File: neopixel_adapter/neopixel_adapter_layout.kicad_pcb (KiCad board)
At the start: 2 copper layers, 91.4 x 81.3 mm, 480 parts, among them J1 Conn_01x02, J2 Conn_01x02

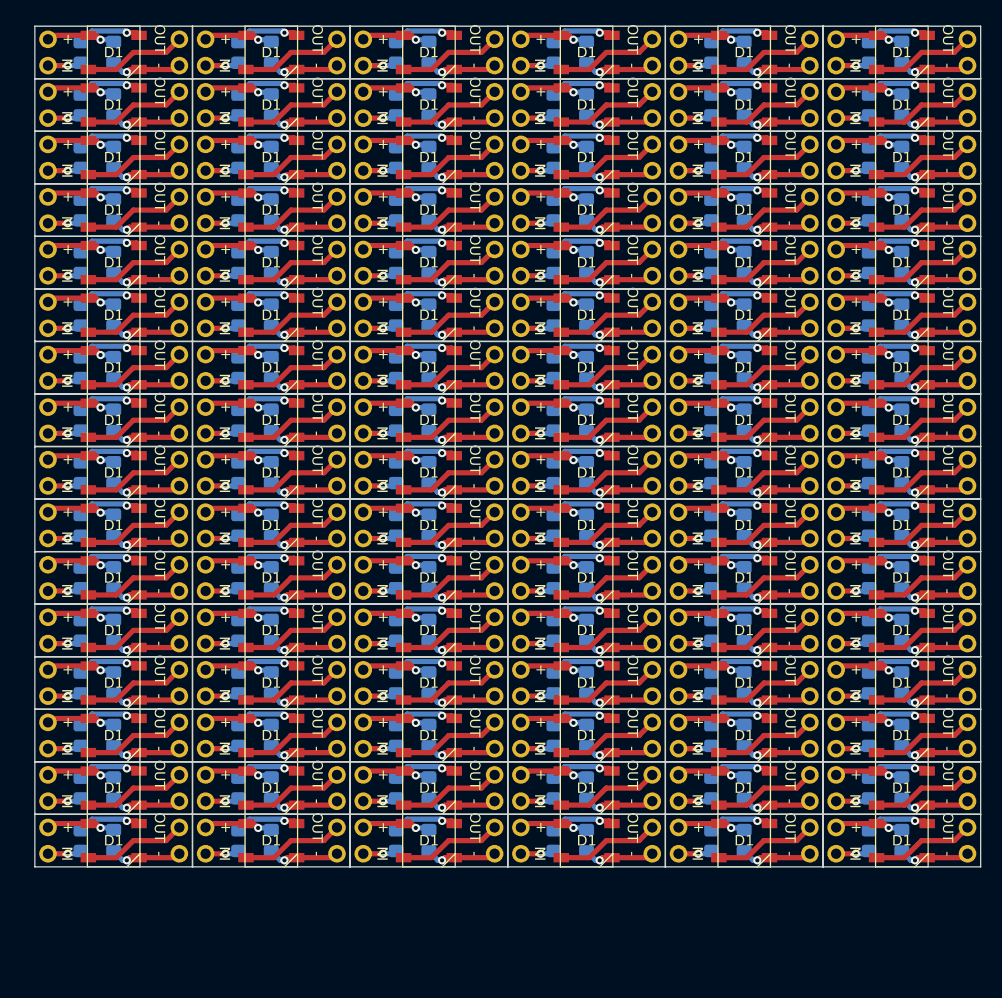
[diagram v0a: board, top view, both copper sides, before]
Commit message: Add .gitignore.
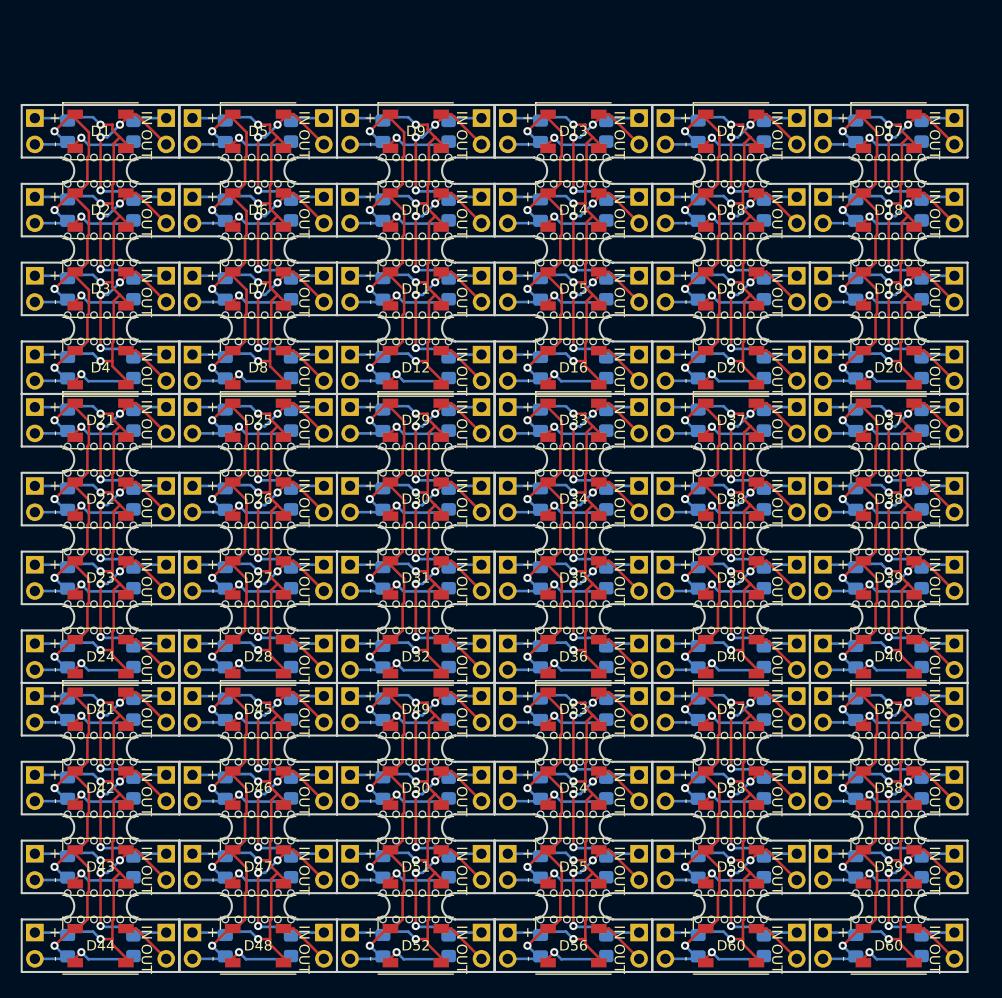
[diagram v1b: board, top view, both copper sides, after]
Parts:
- removed the C1 at (196.8, 68.6)
- removed the C1 at (166.4, 134.6)
- removed the C1 at (151.1, 124.5)
- removed the C1 at (196.8, 144.8)
- removed the C1 at (212.1, 104.1)
- removed the C1 at (181.6, 88.9)
- removed the C1 at (196.8, 139.7)
- removed the C1 at (212.1, 139.7)
- removed the C1 at (212.1, 78.7)
- removed the C1 at (135.9, 94.0)
- removed the C1 at (212.1, 124.5)
- removed the C1 at (181.6, 94.0)
- removed the C1 at (181.6, 129.5)
- removed the C1 at (151.1, 68.6)
- removed the C1 at (166.4, 114.3)
- removed the C1 at (212.1, 83.8)
- removed the C1 at (196.8, 78.7)
- removed the C1 at (166.4, 88.9)
- removed the C1 at (196.8, 109.2)
- removed the C1 at (151.1, 139.7)
- removed the C1 at (212.1, 68.6)
- removed the C1 at (181.6, 73.7)
- removed the C1 at (196.8, 94.0)
- removed the C1 at (166.4, 78.7)
- removed the C1 at (196.8, 119.4)
- removed the C1 at (135.9, 68.6)
- removed the C1 at (212.1, 144.8)
- removed the C1 at (151.1, 119.4)
- removed the C1 at (181.6, 139.7)
- removed the C1 at (181.6, 78.7)
- removed the C1 at (181.6, 124.5)
- removed the C1 at (151.1, 134.6)
- removed the C1 at (212.1, 99.1)
- removed the C1 at (212.1, 119.4)
- removed the C1 at (196.8, 114.3)
- removed the C1 at (212.1, 109.2)
- removed the C1 at (166.4, 109.2)
- removed the C1 at (212.1, 129.5)
- removed the C1 at (135.9, 78.7)
- removed the C1 at (151.1, 78.7)
- removed the C1 at (135.9, 124.5)
- removed the C1 at (196.8, 129.5)
- removed the C1 at (135.9, 144.8)
- removed the C1 at (181.6, 114.3)
- removed the C1 at (181.6, 99.1)
- removed the C1 at (166.4, 124.5)
- removed the C1 at (181.6, 119.4)
- removed the C1 at (166.4, 99.1)
- removed the C1 at (151.1, 88.9)
- removed the C1 at (196.8, 83.8)
- removed the C1 at (166.4, 129.5)
- removed the C1 at (166.4, 139.7)
- removed the C1 at (166.4, 119.4)
- removed the C1 at (181.6, 134.6)
- removed the C1 at (166.4, 83.8)
- removed the C1 at (135.9, 73.7)
- removed the C1 at (151.1, 73.7)
- removed the C1 at (196.8, 88.9)
- removed the C1 at (181.6, 104.1)
- removed the C1 at (135.9, 99.1)
- removed the C1 at (135.9, 109.2)
- removed the C1 at (151.1, 109.2)
- removed the C1 at (166.4, 68.6)
- removed the C1 at (196.8, 134.6)
- removed the C1 at (212.1, 88.9)
- removed the C1 at (212.1, 114.3)
- removed the C1 at (151.1, 99.1)
- removed the C1 at (151.1, 94.0)
- removed the C1 at (135.9, 139.7)
- removed the C1 at (151.1, 144.8)
- removed the C1 at (151.1, 83.8)
- removed the C1 at (135.9, 134.6)
- removed the C1 at (135.9, 83.8)
- removed the C1 at (196.8, 124.5)
- removed the C1 at (135.9, 88.9)
- removed the C1 at (151.1, 129.5)
- removed the C1 at (181.6, 144.8)
- removed the C1 at (135.9, 129.5)
- removed the C1 at (212.1, 94.0)
- removed the C1 at (212.1, 134.6)
- removed the C1 at (212.1, 73.7)
- removed the C1 at (135.9, 119.4)
- removed the C1 at (166.4, 94.0)
- removed the C1 at (181.6, 83.8)
- removed the C1 at (166.4, 144.8)
- removed the C1 at (151.1, 114.3)
- removed the C1 at (166.4, 104.1)
- removed the C1 at (181.6, 109.2)
- removed the C1 at (135.9, 114.3)
- removed the C1 at (151.1, 104.1)
- removed the C1 at (196.8, 99.1)
- removed the C1 at (196.8, 73.7)
- removed the C1 at (196.8, 104.1)
- removed the C1 at (181.6, 68.6)
- removed the C1 at (166.4, 73.7)
- removed the C1 at (135.9, 104.1)
- removed the D1 at (166.4, 68.6)
- removed the D1 at (135.9, 94.0)
- removed the D1 at (181.6, 88.9)
- removed the D1 at (135.9, 139.7)
- removed the D1 at (135.9, 124.5)
- removed the D1 at (181.6, 94.0)
- removed the D1 at (196.8, 144.8)
- removed the D1 at (181.6, 134.6)
- removed the D1 at (135.9, 129.5)
- removed the D1 at (166.4, 78.7)
- removed the D1 at (135.9, 134.6)
- removed the D1 at (135.9, 99.1)
- removed the D1 at (135.9, 88.9)
- removed the D1 at (166.4, 139.7)
- removed the D1 at (196.8, 139.7)
- removed the D1 at (212.1, 139.7)
- removed the D1 at (151.1, 78.7)
- removed the D1 at (196.8, 73.7)
- removed the D1 at (166.4, 109.2)
- removed the D1 at (166.4, 94.0)
- removed the D1 at (166.4, 114.3)
- removed the D1 at (166.4, 119.4)
- removed the D1 at (166.4, 83.8)
- removed the D1 at (181.6, 99.1)
- removed the D1 at (196.8, 114.3)
- removed the D1 at (196.8, 68.6)
- removed the D1 at (181.6, 109.2)
- removed the D1 at (181.6, 144.8)
- removed the D1 at (181.6, 78.7)
- removed the D1 at (212.1, 144.8)
- removed the D1 at (151.1, 68.6)
- removed the D1 at (196.8, 124.5)
- removed the D1 at (212.1, 119.4)
- removed the D1 at (135.9, 73.7)
- removed the D1 at (212.1, 68.6)
- removed the D1 at (151.1, 129.5)
- removed the D1 at (196.8, 104.1)
- removed the D1 at (151.1, 83.8)
- removed the D1 at (151.1, 104.1)
- removed the D1 at (181.6, 114.3)
- removed the D1 at (181.6, 73.7)
- removed the D1 at (212.1, 109.2)
- removed the D1 at (135.9, 104.1)
- removed the D1 at (166.4, 129.5)
- removed the D1 at (196.8, 94.0)
- removed the D1 at (196.8, 88.9)
- removed the D1 at (166.4, 144.8)
- removed the D1 at (196.8, 83.8)
- removed the D1 at (166.4, 73.7)
- removed the D1 at (212.1, 114.3)
- removed the D1 at (135.9, 68.6)
- removed the D1 at (181.6, 83.8)
- removed the D1 at (135.9, 144.8)
- removed the D1 at (196.8, 119.4)
- removed the D1 at (212.1, 104.1)
- removed the D1 at (196.8, 109.2)
- removed the D1 at (151.1, 94.0)
- removed the D1 at (212.1, 88.9)
- removed the D1 at (196.8, 129.5)
- removed the D1 at (151.1, 114.3)
- removed the D1 at (151.1, 119.4)
- removed the D1 at (135.9, 114.3)
- removed the D1 at (181.6, 119.4)
- removed the D1 at (151.1, 134.6)
- removed the D1 at (212.1, 124.5)
- removed the D1 at (166.4, 88.9)
- removed the D1 at (181.6, 104.1)
- removed the D1 at (212.1, 73.7)
- removed the D1 at (166.4, 99.1)
- removed the D1 at (181.6, 139.7)
- removed the D1 at (212.1, 83.8)
- removed the D1 at (151.1, 139.7)
- removed the D1 at (135.9, 83.8)
- removed the D1 at (212.1, 78.7)
- removed the D1 at (151.1, 109.2)
- removed the D1 at (166.4, 104.1)
- removed the D1 at (212.1, 129.5)
- removed the D1 at (151.1, 144.8)
- removed the D1 at (151.1, 124.5)
- removed the D1 at (135.9, 109.2)
- removed the D1 at (151.1, 88.9)
- removed the D1 at (151.1, 99.1)
- removed the D1 at (135.9, 78.7)
- removed the D1 at (196.8, 134.6)
- removed the D1 at (212.1, 134.6)
- removed the D1 at (181.6, 68.6)
- removed the D1 at (181.6, 129.5)
- removed the D1 at (135.9, 119.4)
- removed the D1 at (212.1, 99.1)
- removed the D1 at (212.1, 94.0)
- removed the D1 at (196.8, 78.7)
- removed the D1 at (181.6, 124.5)
- removed the D1 at (166.4, 134.6)
- removed the D1 at (151.1, 73.7)
- removed the D1 at (166.4, 124.5)
- removed the D1 at (196.8, 99.1)
- removed the J1 at (190.5, 143.5)
- removed the J1 at (205.7, 92.7)
- removed the J1 at (160.0, 128.3)
- removed the J1 at (129.5, 82.5)
- removed the J1 at (175.3, 118.1)
- removed the J1 at (129.5, 118.1)
- removed the J1 at (190.5, 108.0)
- removed the J1 at (144.8, 102.9)
- removed the J1 at (205.7, 143.5)
- removed the J1 at (175.3, 123.2)
- removed the J1 at (205.7, 113.0)
- removed the J1 at (205.7, 77.5)
- removed the J1 at (175.3, 143.5)
- removed the J1 at (190.5, 97.8)
- removed the J1 at (160.0, 97.8)
- removed the J1 at (205.7, 108.0)
- removed the J1 at (129.5, 72.4)
- removed the J1 at (129.5, 92.7)
- removed the J1 at (144.8, 113.0)
- removed the J1 at (175.3, 128.3)
- removed the J1 at (129.5, 123.2)
- removed the J1 at (160.0, 87.6)
- removed the J1 at (160.0, 92.7)
- removed the J1 at (129.5, 128.3)
- removed the J1 at (205.7, 82.5)
- removed the J1 at (144.8, 77.5)
- removed the J1 at (144.8, 87.6)
- removed the J1 at (205.7, 97.8)
- removed the J1 at (190.5, 72.4)
- removed the J1 at (205.7, 138.4)
- removed the J1 at (175.3, 113.0)
- removed the J1 at (190.5, 102.9)
- removed the J1 at (144.8, 128.3)
- removed the J1 at (144.8, 92.7)
- removed the J1 at (160.0, 67.3)
- removed the J1 at (190.5, 123.2)
- removed the J1 at (144.8, 82.5)
- removed the J1 at (129.5, 143.5)
- removed the J1 at (129.5, 108.0)
- removed the J1 at (190.5, 138.4)
- removed the J1 at (175.3, 138.4)
- removed the J1 at (190.5, 67.3)
- removed the J1 at (205.7, 128.3)
- removed the J1 at (175.3, 82.5)
- removed the J1 at (129.5, 102.9)
- removed the J1 at (190.5, 92.7)
- removed the J1 at (205.7, 118.1)
- removed the J1 at (190.5, 113.0)
- removed the J1 at (144.8, 123.2)
- removed the J1 at (160.0, 113.0)
- removed the J1 at (175.3, 108.0)
- removed the J1 at (190.5, 133.3)
- removed the J1 at (190.5, 87.6)
- removed the J1 at (175.3, 87.6)
- removed the J1 at (160.0, 123.2)
- removed the J1 at (205.7, 133.3)
- removed the J1 at (160.0, 72.4)
- removed the J1 at (144.8, 108.0)
- removed the J1 at (175.3, 67.3)
- removed the J1 at (129.5, 138.4)
- removed the J1 at (205.7, 67.3)
- removed the J1 at (205.7, 72.4)
- removed the J1 at (160.0, 118.1)
- removed the J1 at (144.8, 72.4)
- removed the J1 at (129.5, 113.0)
- removed the J1 at (175.3, 97.8)
- removed the J1 at (144.8, 143.5)
- removed the J1 at (160.0, 108.0)
- removed the J1 at (190.5, 77.5)
- removed the J1 at (175.3, 92.7)
- removed the J1 at (205.7, 102.9)
- removed the J1 at (129.5, 133.3)
- removed the J1 at (175.3, 102.9)
- removed the J1 at (160.0, 82.5)
- removed the J1 at (129.5, 97.8)
- removed the J1 at (144.8, 118.1)
- removed the J1 at (175.3, 133.3)
- removed the J1 at (144.8, 133.3)
- removed the J1 at (190.5, 128.3)
- removed the J1 at (175.3, 77.5)
- removed the J1 at (190.5, 118.1)
- removed the J1 at (160.0, 102.9)
- removed the J1 at (205.7, 123.2)
- removed the J1 at (129.5, 77.5)
- removed the J1 at (129.5, 87.6)
- removed the J1 at (160.0, 77.5)
- removed the J1 at (129.5, 67.3)
- removed the J1 at (160.0, 138.4)
- removed the J1 at (160.0, 133.3)
- removed the J1 at (144.8, 97.8)
- removed the J1 at (175.3, 72.4)
- removed the J1 at (144.8, 67.3)
- removed the J1 at (160.0, 143.5)
- removed the J1 at (190.5, 82.5)
- removed the J1 at (144.8, 138.4)
- removed the J1 at (205.7, 87.6)
- removed the J2 at (172.7, 133.3)
- removed the J2 at (142.2, 97.8)
- removed the J2 at (218.4, 77.5)
- removed the J2 at (203.2, 97.8)
- removed the J2 at (172.7, 128.3)
- removed the J2 at (142.2, 123.2)
- removed the J2 at (142.2, 92.7)
- removed the J2 at (188.0, 67.3)
- removed the J2 at (157.5, 97.8)
- removed the J2 at (218.4, 102.9)
- removed the J2 at (157.5, 128.3)
- removed the J2 at (172.7, 108.0)
- removed the J2 at (172.7, 138.4)
- removed the J2 at (157.5, 143.5)
- removed the J2 at (157.5, 102.9)
- removed the J2 at (142.2, 138.4)
- removed the J2 at (157.5, 92.7)
- removed the J2 at (218.4, 138.4)
- removed the J2 at (218.4, 118.1)
- removed the J2 at (188.0, 72.4)
- removed the J2 at (218.4, 128.3)
- removed the J2 at (142.2, 82.5)
- removed the J2 at (157.5, 87.6)
- removed the J2 at (218.4, 82.5)
- removed the J2 at (172.7, 92.7)
- removed the J2 at (188.0, 97.8)
- removed the J2 at (218.4, 92.7)
- removed the J2 at (188.0, 138.4)
- removed the J2 at (172.7, 72.4)
- removed the J2 at (188.0, 143.5)
- removed the J2 at (203.2, 143.5)
- removed the J2 at (172.7, 82.5)
- removed the J2 at (142.2, 128.3)
- removed the J2 at (218.4, 123.2)
- removed the J2 at (172.7, 113.0)
- removed the J2 at (188.0, 92.7)
- removed the J2 at (203.2, 113.0)
- removed the J2 at (172.7, 87.6)
- removed the J2 at (203.2, 123.2)
- removed the J2 at (157.5, 113.0)
- removed the J2 at (157.5, 77.5)
- removed the J2 at (203.2, 77.5)
- removed the J2 at (203.2, 118.1)
- removed the J2 at (172.7, 77.5)
- removed the J2 at (142.2, 87.6)
- removed the J2 at (203.2, 138.4)
- removed the J2 at (218.4, 67.3)
- removed the J2 at (188.0, 108.0)
- removed the J2 at (188.0, 123.2)
- removed the J2 at (142.2, 113.0)
- removed the J2 at (218.4, 133.3)
- removed the J2 at (203.2, 108.0)
- removed the J2 at (172.7, 67.3)
- removed the J2 at (142.2, 72.4)
- removed the J2 at (203.2, 72.4)
- removed the J2 at (157.5, 108.0)
- removed the J2 at (142.2, 108.0)
- removed the J2 at (188.0, 128.3)
- removed the J2 at (203.2, 128.3)
- removed the J2 at (188.0, 133.3)
- removed the J2 at (157.5, 133.3)
- removed the J2 at (172.7, 118.1)
- removed the J2 at (188.0, 82.5)
- removed the J2 at (218.4, 97.8)
- removed the J2 at (203.2, 92.7)
- removed the J2 at (157.5, 82.5)
- removed the J2 at (218.4, 143.5)
- removed the J2 at (218.4, 87.6)
- removed the J2 at (142.2, 102.9)
- removed the J2 at (172.7, 143.5)
- removed the J2 at (188.0, 118.1)
- removed the J2 at (203.2, 133.3)
- removed the J2 at (157.5, 118.1)
- removed the J2 at (188.0, 102.9)
- removed the J2 at (172.7, 97.8)
- removed the J2 at (218.4, 113.0)
- removed the J2 at (157.5, 138.4)
- removed the J2 at (157.5, 72.4)
- removed the J2 at (142.2, 143.5)
- removed the J2 at (157.5, 123.2)
- removed the J2 at (218.4, 108.0)
- removed the J2 at (142.2, 133.3)
- removed the J2 at (203.2, 67.3)
- removed the J2 at (157.5, 67.3)
- removed the J2 at (203.2, 87.6)
- removed the J2 at (188.0, 77.5)
- removed the J2 at (172.7, 102.9)
- removed the J2 at (203.2, 102.9)
- removed the J2 at (218.4, 72.4)
- removed the J2 at (203.2, 82.5)
- removed the J2 at (142.2, 67.3)
- removed the J2 at (142.2, 77.5)
- removed the J2 at (172.7, 123.2)
- removed the J2 at (188.0, 113.0)
- removed the J2 at (142.2, 118.1)
- removed the J2 at (188.0, 87.6)
- removed the R1 at (178.4, 114.3)
- removed the R1 at (132.7, 99.1)
- removed the R1 at (193.7, 124.5)
- removed the R1 at (148.0, 94.0)
- removed the R1 at (178.4, 83.8)
- removed the R1 at (193.7, 94.0)
- removed the R1 at (163.2, 78.7)
- removed the R1 at (132.7, 114.3)
- removed the R1 at (178.4, 73.7)
- removed the R1 at (163.2, 144.8)
- removed the R1 at (193.7, 139.7)
- removed the R1 at (132.7, 88.9)
- removed the R1 at (148.0, 73.7)
- removed the R1 at (148.0, 68.6)
- removed the R1 at (178.4, 99.1)
- removed the R1 at (163.2, 104.1)
- removed the R1 at (193.7, 83.8)
- removed the R1 at (193.7, 114.3)
- removed the R1 at (178.4, 88.9)
- removed the R1 at (148.0, 134.6)
- removed the R1 at (132.7, 124.5)
- removed the R1 at (132.7, 68.6)
- removed the R1 at (178.4, 78.7)
- removed the R1 at (208.9, 83.8)
- removed the R1 at (208.9, 99.1)
- removed the R1 at (132.7, 94.0)
- removed the R1 at (208.9, 129.5)
- removed the R1 at (178.4, 144.8)
- removed the R1 at (132.7, 104.1)
- removed the R1 at (178.4, 134.6)
- removed the R1 at (193.7, 119.4)
- removed the R1 at (193.7, 134.6)
- removed the R1 at (208.9, 88.9)
- removed the R1 at (178.4, 139.7)
- removed the R1 at (163.2, 114.3)
- removed the R1 at (178.4, 124.5)
- removed the R1 at (132.7, 144.8)
- removed the R1 at (193.7, 144.8)
- removed the R1 at (163.2, 124.5)
- removed the R1 at (208.9, 119.4)
- removed the R1 at (178.4, 129.5)
- removed the R1 at (163.2, 73.7)
- removed the R1 at (163.2, 134.6)
- removed the R1 at (163.2, 83.8)
- removed the R1 at (208.9, 73.7)
- removed the R1 at (148.0, 124.5)
- removed the R1 at (178.4, 94.0)
- removed the R1 at (148.0, 114.3)
- removed the R1 at (163.2, 88.9)
- removed the R1 at (163.2, 129.5)
- removed the R1 at (208.9, 109.2)
- removed the R1 at (193.7, 109.2)
- removed the R1 at (178.4, 119.4)
- removed the R1 at (148.0, 129.5)
- removed the R1 at (193.7, 104.1)
- removed the R1 at (132.7, 73.7)
- removed the R1 at (148.0, 139.7)
- removed the R1 at (148.0, 99.1)
- removed the R1 at (208.9, 139.7)
- removed the R1 at (148.0, 104.1)
- removed the R1 at (178.4, 109.2)
- removed the R1 at (208.9, 68.6)
- removed the R1 at (193.7, 99.1)
- removed the R1 at (163.2, 68.6)
- removed the R1 at (193.7, 129.5)
- removed the R1 at (132.7, 109.2)
- removed the R1 at (193.7, 88.9)
- removed the R1 at (132.7, 129.5)
- removed the R1 at (132.7, 139.7)
- removed the R1 at (208.9, 134.6)
- removed the R1 at (148.0, 119.4)
- removed the R1 at (163.2, 119.4)
- removed the R1 at (193.7, 68.6)
- removed the R1 at (132.7, 78.7)
- removed the R1 at (193.7, 78.7)
- removed the R1 at (163.2, 94.0)
- removed the R1 at (178.4, 68.6)
- removed the R1 at (148.0, 78.7)
- removed the R1 at (163.2, 139.7)
- removed the R1 at (163.2, 109.2)
- removed the R1 at (178.4, 104.1)
- removed the R1 at (132.7, 83.8)
- removed the R1 at (208.9, 94.0)
- removed the R1 at (163.2, 99.1)
- removed the R1 at (148.0, 88.9)
- removed the R1 at (208.9, 124.5)
- removed the R1 at (148.0, 144.8)
- removed the R1 at (208.9, 144.8)
- removed the R1 at (132.7, 134.6)
- removed the R1 at (208.9, 78.7)
- removed the R1 at (148.0, 109.2)
- removed the R1 at (208.9, 104.1)
- removed the R1 at (132.7, 119.4)
- removed the R1 at (208.9, 114.3)
- removed the R1 at (193.7, 73.7)
- removed the R1 at (148.0, 83.8)
- added C1: 0.1uF, Capacitor_SMD:C_0805_2012Metric_Pad1.18x1.45mm_HandSolder, B.Cu at (131.4, 76.2)
- added C10: 0.1uF, Capacitor_SMD:C_0805_2012Metric_Pad1.18x1.45mm_HandSolder, B.Cu at (161.9, 83.8)
- added C11: 0.1uF, Capacitor_SMD:C_0805_2012Metric_Pad1.18x1.45mm_HandSolder, B.Cu at (161.9, 91.4)
- added C12: 0.1uF, Capacitor_SMD:C_0805_2012Metric_Pad1.18x1.45mm_HandSolder, B.Cu at (161.9, 99.1)
- added C13: 0.1uF, Capacitor_SMD:C_0805_2012Metric_Pad1.18x1.45mm_HandSolder, B.Cu at (177.2, 76.2)
- added C14: 0.1uF, Capacitor_SMD:C_0805_2012Metric_Pad1.18x1.45mm_HandSolder, B.Cu at (177.2, 83.8)
- added C15: 0.1uF, Capacitor_SMD:C_0805_2012Metric_Pad1.18x1.45mm_HandSolder, B.Cu at (177.2, 91.4)
- added C16: 0.1uF, Capacitor_SMD:C_0805_2012Metric_Pad1.18x1.45mm_HandSolder, B.Cu at (177.2, 99.1)
- added C17: 0.1uF, Capacitor_SMD:C_0805_2012Metric_Pad1.18x1.45mm_HandSolder, B.Cu at (207.6, 76.2)
- added C17: 0.1uF, Capacitor_SMD:C_0805_2012Metric_Pad1.18x1.45mm_HandSolder, B.Cu at (192.4, 76.2)
- added C18: 0.1uF, Capacitor_SMD:C_0805_2012Metric_Pad1.18x1.45mm_HandSolder, B.Cu at (192.4, 83.8)
- added C18: 0.1uF, Capacitor_SMD:C_0805_2012Metric_Pad1.18x1.45mm_HandSolder, B.Cu at (207.6, 83.8)
- added C19: 0.1uF, Capacitor_SMD:C_0805_2012Metric_Pad1.18x1.45mm_HandSolder, B.Cu at (207.6, 91.4)
- added C19: 0.1uF, Capacitor_SMD:C_0805_2012Metric_Pad1.18x1.45mm_HandSolder, B.Cu at (192.4, 91.4)
- added C2: 0.1uF, Capacitor_SMD:C_0805_2012Metric_Pad1.18x1.45mm_HandSolder, B.Cu at (131.4, 83.8)
- added C20: 0.1uF, Capacitor_SMD:C_0805_2012Metric_Pad1.18x1.45mm_HandSolder, B.Cu at (207.6, 99.1)
- added C20: 0.1uF, Capacitor_SMD:C_0805_2012Metric_Pad1.18x1.45mm_HandSolder, B.Cu at (192.4, 99.1)
- added C21: 0.1uF, Capacitor_SMD:C_0805_2012Metric_Pad1.18x1.45mm_HandSolder, B.Cu at (131.4, 104.1)
- added C22: 0.1uF, Capacitor_SMD:C_0805_2012Metric_Pad1.18x1.45mm_HandSolder, B.Cu at (131.4, 111.8)
- added C23: 0.1uF, Capacitor_SMD:C_0805_2012Metric_Pad1.18x1.45mm_HandSolder, B.Cu at (131.4, 119.4)
- added C24: 0.1uF, Capacitor_SMD:C_0805_2012Metric_Pad1.18x1.45mm_HandSolder, B.Cu at (131.4, 127.0)
- added C25: 0.1uF, Capacitor_SMD:C_0805_2012Metric_Pad1.18x1.45mm_HandSolder, B.Cu at (146.7, 104.1)
- added C26: 0.1uF, Capacitor_SMD:C_0805_2012Metric_Pad1.18x1.45mm_HandSolder, B.Cu at (146.7, 111.8)
- added C27: 0.1uF, Capacitor_SMD:C_0805_2012Metric_Pad1.18x1.45mm_HandSolder, B.Cu at (146.7, 119.4)
- added C28: 0.1uF, Capacitor_SMD:C_0805_2012Metric_Pad1.18x1.45mm_HandSolder, B.Cu at (146.7, 127.0)
- added C29: 0.1uF, Capacitor_SMD:C_0805_2012Metric_Pad1.18x1.45mm_HandSolder, B.Cu at (161.9, 104.1)
- added C3: 0.1uF, Capacitor_SMD:C_0805_2012Metric_Pad1.18x1.45mm_HandSolder, B.Cu at (131.4, 91.4)
- added C30: 0.1uF, Capacitor_SMD:C_0805_2012Metric_Pad1.18x1.45mm_HandSolder, B.Cu at (161.9, 111.8)
- added C31: 0.1uF, Capacitor_SMD:C_0805_2012Metric_Pad1.18x1.45mm_HandSolder, B.Cu at (161.9, 119.4)
- added C32: 0.1uF, Capacitor_SMD:C_0805_2012Metric_Pad1.18x1.45mm_HandSolder, B.Cu at (161.9, 127.0)
- added C33: 0.1uF, Capacitor_SMD:C_0805_2012Metric_Pad1.18x1.45mm_HandSolder, B.Cu at (177.2, 104.1)
- added C34: 0.1uF, Capacitor_SMD:C_0805_2012Metric_Pad1.18x1.45mm_HandSolder, B.Cu at (177.2, 111.8)
- added C35: 0.1uF, Capacitor_SMD:C_0805_2012Metric_Pad1.18x1.45mm_HandSolder, B.Cu at (177.2, 119.4)
- added C36: 0.1uF, Capacitor_SMD:C_0805_2012Metric_Pad1.18x1.45mm_HandSolder, B.Cu at (177.2, 127.0)
- added C37: 0.1uF, Capacitor_SMD:C_0805_2012Metric_Pad1.18x1.45mm_HandSolder, B.Cu at (207.6, 104.1)
- added C37: 0.1uF, Capacitor_SMD:C_0805_2012Metric_Pad1.18x1.45mm_HandSolder, B.Cu at (192.4, 104.1)
- added C38: 0.1uF, Capacitor_SMD:C_0805_2012Metric_Pad1.18x1.45mm_HandSolder, B.Cu at (192.4, 111.8)
- added C38: 0.1uF, Capacitor_SMD:C_0805_2012Metric_Pad1.18x1.45mm_HandSolder, B.Cu at (207.6, 111.8)
- added C39: 0.1uF, Capacitor_SMD:C_0805_2012Metric_Pad1.18x1.45mm_HandSolder, B.Cu at (192.4, 119.4)
- added C39: 0.1uF, Capacitor_SMD:C_0805_2012Metric_Pad1.18x1.45mm_HandSolder, B.Cu at (207.6, 119.4)
- added C4: 0.1uF, Capacitor_SMD:C_0805_2012Metric_Pad1.18x1.45mm_HandSolder, B.Cu at (131.4, 99.1)
- added C40: 0.1uF, Capacitor_SMD:C_0805_2012Metric_Pad1.18x1.45mm_HandSolder, B.Cu at (207.6, 127.0)
- added C40: 0.1uF, Capacitor_SMD:C_0805_2012Metric_Pad1.18x1.45mm_HandSolder, B.Cu at (192.4, 127.0)
- added C41: 0.1uF, Capacitor_SMD:C_0805_2012Metric_Pad1.18x1.45mm_HandSolder, B.Cu at (131.4, 132.1)
- added C42: 0.1uF, Capacitor_SMD:C_0805_2012Metric_Pad1.18x1.45mm_HandSolder, B.Cu at (131.4, 139.7)
- added C43: 0.1uF, Capacitor_SMD:C_0805_2012Metric_Pad1.18x1.45mm_HandSolder, B.Cu at (131.4, 147.3)
- added C44: 0.1uF, Capacitor_SMD:C_0805_2012Metric_Pad1.18x1.45mm_HandSolder, B.Cu at (131.4, 154.9)
- added C45: 0.1uF, Capacitor_SMD:C_0805_2012Metric_Pad1.18x1.45mm_HandSolder, B.Cu at (146.7, 132.1)
- added C46: 0.1uF, Capacitor_SMD:C_0805_2012Metric_Pad1.18x1.45mm_HandSolder, B.Cu at (146.7, 139.7)
- added C47: 0.1uF, Capacitor_SMD:C_0805_2012Metric_Pad1.18x1.45mm_HandSolder, B.Cu at (146.7, 147.3)
- added C48: 0.1uF, Capacitor_SMD:C_0805_2012Metric_Pad1.18x1.45mm_HandSolder, B.Cu at (146.7, 154.9)
- added C49: 0.1uF, Capacitor_SMD:C_0805_2012Metric_Pad1.18x1.45mm_HandSolder, B.Cu at (161.9, 132.1)
- added C5: 0.1uF, Capacitor_SMD:C_0805_2012Metric_Pad1.18x1.45mm_HandSolder, B.Cu at (146.7, 76.2)
- added C50: 0.1uF, Capacitor_SMD:C_0805_2012Metric_Pad1.18x1.45mm_HandSolder, B.Cu at (161.9, 139.7)
- added C51: 0.1uF, Capacitor_SMD:C_0805_2012Metric_Pad1.18x1.45mm_HandSolder, B.Cu at (161.9, 147.3)
- added C52: 0.1uF, Capacitor_SMD:C_0805_2012Metric_Pad1.18x1.45mm_HandSolder, B.Cu at (161.9, 154.9)
- added C53: 0.1uF, Capacitor_SMD:C_0805_2012Metric_Pad1.18x1.45mm_HandSolder, B.Cu at (177.2, 132.1)
- added C54: 0.1uF, Capacitor_SMD:C_0805_2012Metric_Pad1.18x1.45mm_HandSolder, B.Cu at (177.2, 139.7)
- added C55: 0.1uF, Capacitor_SMD:C_0805_2012Metric_Pad1.18x1.45mm_HandSolder, B.Cu at (177.2, 147.3)
- added C56: 0.1uF, Capacitor_SMD:C_0805_2012Metric_Pad1.18x1.45mm_HandSolder, B.Cu at (177.2, 154.9)
- added C57: 0.1uF, Capacitor_SMD:C_0805_2012Metric_Pad1.18x1.45mm_HandSolder, B.Cu at (207.6, 132.1)
- added C57: 0.1uF, Capacitor_SMD:C_0805_2012Metric_Pad1.18x1.45mm_HandSolder, B.Cu at (192.4, 132.1)
- added C58: 0.1uF, Capacitor_SMD:C_0805_2012Metric_Pad1.18x1.45mm_HandSolder, B.Cu at (192.4, 139.7)
- added C58: 0.1uF, Capacitor_SMD:C_0805_2012Metric_Pad1.18x1.45mm_HandSolder, B.Cu at (207.6, 139.7)
- added C59: 0.1uF, Capacitor_SMD:C_0805_2012Metric_Pad1.18x1.45mm_HandSolder, B.Cu at (207.6, 147.3)
- added C59: 0.1uF, Capacitor_SMD:C_0805_2012Metric_Pad1.18x1.45mm_HandSolder, B.Cu at (192.4, 147.3)
- added C6: 0.1uF, Capacitor_SMD:C_0805_2012Metric_Pad1.18x1.45mm_HandSolder, B.Cu at (146.7, 83.8)
- added C60: 0.1uF, Capacitor_SMD:C_0805_2012Metric_Pad1.18x1.45mm_HandSolder, B.Cu at (207.6, 154.9)
- added C60: 0.1uF, Capacitor_SMD:C_0805_2012Metric_Pad1.18x1.45mm_HandSolder, B.Cu at (192.4, 154.9)
- added C7: 0.1uF, Capacitor_SMD:C_0805_2012Metric_Pad1.18x1.45mm_HandSolder, B.Cu at (146.7, 91.4)
- added C8: 0.1uF, Capacitor_SMD:C_0805_2012Metric_Pad1.18x1.45mm_HandSolder, B.Cu at (146.7, 99.1)
- added C9: 0.1uF, Capacitor_SMD:C_0805_2012Metric_Pad1.18x1.45mm_HandSolder, B.Cu at (161.9, 76.2)
- added D1: WS2812B, LED_SMD:LED_WS2812B_PLCC4_5.0x5.0mm_P3.2mm, F.Cu at (134.6, 76.2)
- added D10: WS2812B, LED_SMD:LED_WS2812B_PLCC4_5.0x5.0mm_P3.2mm, F.Cu at (165.1, 83.8)
- added D11: WS2812B, LED_SMD:LED_WS2812B_PLCC4_5.0x5.0mm_P3.2mm, F.Cu at (165.1, 91.4)
- added D12: WS2812B, LED_SMD:LED_WS2812B_PLCC4_5.0x5.0mm_P3.2mm, F.Cu at (165.1, 99.1)
- added D13: WS2812B, LED_SMD:LED_WS2812B_PLCC4_5.0x5.0mm_P3.2mm, F.Cu at (180.3, 76.2)
- added D14: WS2812B, LED_SMD:LED_WS2812B_PLCC4_5.0x5.0mm_P3.2mm, F.Cu at (180.3, 83.8)
- added D15: WS2812B, LED_SMD:LED_WS2812B_PLCC4_5.0x5.0mm_P3.2mm, F.Cu at (180.3, 91.4)
- added D16: WS2812B, LED_SMD:LED_WS2812B_PLCC4_5.0x5.0mm_P3.2mm, F.Cu at (180.3, 99.1)
- added D17: WS2812B, LED_SMD:LED_WS2812B_PLCC4_5.0x5.0mm_P3.2mm, F.Cu at (195.6, 76.2)
- added D17: WS2812B, LED_SMD:LED_WS2812B_PLCC4_5.0x5.0mm_P3.2mm, F.Cu at (210.8, 76.2)
- added D18: WS2812B, LED_SMD:LED_WS2812B_PLCC4_5.0x5.0mm_P3.2mm, F.Cu at (195.6, 83.8)
- added D18: WS2812B, LED_SMD:LED_WS2812B_PLCC4_5.0x5.0mm_P3.2mm, F.Cu at (210.8, 83.8)
- added D19: WS2812B, LED_SMD:LED_WS2812B_PLCC4_5.0x5.0mm_P3.2mm, F.Cu at (195.6, 91.4)
- added D19: WS2812B, LED_SMD:LED_WS2812B_PLCC4_5.0x5.0mm_P3.2mm, F.Cu at (210.8, 91.4)
- added D2: WS2812B, LED_SMD:LED_WS2812B_PLCC4_5.0x5.0mm_P3.2mm, F.Cu at (134.6, 83.8)
- added D20: WS2812B, LED_SMD:LED_WS2812B_PLCC4_5.0x5.0mm_P3.2mm, F.Cu at (195.6, 99.1)
- added D20: WS2812B, LED_SMD:LED_WS2812B_PLCC4_5.0x5.0mm_P3.2mm, F.Cu at (210.8, 99.1)
- added D21: WS2812B, LED_SMD:LED_WS2812B_PLCC4_5.0x5.0mm_P3.2mm, F.Cu at (134.6, 104.1)
- added D22: WS2812B, LED_SMD:LED_WS2812B_PLCC4_5.0x5.0mm_P3.2mm, F.Cu at (134.6, 111.8)
- added D23: WS2812B, LED_SMD:LED_WS2812B_PLCC4_5.0x5.0mm_P3.2mm, F.Cu at (134.6, 119.4)
- added D24: WS2812B, LED_SMD:LED_WS2812B_PLCC4_5.0x5.0mm_P3.2mm, F.Cu at (134.6, 127.0)
- added D25: WS2812B, LED_SMD:LED_WS2812B_PLCC4_5.0x5.0mm_P3.2mm, F.Cu at (149.9, 104.1)
- added D26: WS2812B, LED_SMD:LED_WS2812B_PLCC4_5.0x5.0mm_P3.2mm, F.Cu at (149.9, 111.8)
- added D27: WS2812B, LED_SMD:LED_WS2812B_PLCC4_5.0x5.0mm_P3.2mm, F.Cu at (149.9, 119.4)
- added D28: WS2812B, LED_SMD:LED_WS2812B_PLCC4_5.0x5.0mm_P3.2mm, F.Cu at (149.9, 127.0)
- added D29: WS2812B, LED_SMD:LED_WS2812B_PLCC4_5.0x5.0mm_P3.2mm, F.Cu at (165.1, 104.1)
- added D3: WS2812B, LED_SMD:LED_WS2812B_PLCC4_5.0x5.0mm_P3.2mm, F.Cu at (134.6, 91.4)
- added D30: WS2812B, LED_SMD:LED_WS2812B_PLCC4_5.0x5.0mm_P3.2mm, F.Cu at (165.1, 111.8)
- added D31: WS2812B, LED_SMD:LED_WS2812B_PLCC4_5.0x5.0mm_P3.2mm, F.Cu at (165.1, 119.4)
- added D32: WS2812B, LED_SMD:LED_WS2812B_PLCC4_5.0x5.0mm_P3.2mm, F.Cu at (165.1, 127.0)
- added D33: WS2812B, LED_SMD:LED_WS2812B_PLCC4_5.0x5.0mm_P3.2mm, F.Cu at (180.3, 104.1)
- added D34: WS2812B, LED_SMD:LED_WS2812B_PLCC4_5.0x5.0mm_P3.2mm, F.Cu at (180.3, 111.8)
- added D35: WS2812B, LED_SMD:LED_WS2812B_PLCC4_5.0x5.0mm_P3.2mm, F.Cu at (180.3, 119.4)
- added D36: WS2812B, LED_SMD:LED_WS2812B_PLCC4_5.0x5.0mm_P3.2mm, F.Cu at (180.3, 127.0)
- added D37: WS2812B, LED_SMD:LED_WS2812B_PLCC4_5.0x5.0mm_P3.2mm, F.Cu at (195.6, 104.1)
- added D37: WS2812B, LED_SMD:LED_WS2812B_PLCC4_5.0x5.0mm_P3.2mm, F.Cu at (210.8, 104.1)
- added D38: WS2812B, LED_SMD:LED_WS2812B_PLCC4_5.0x5.0mm_P3.2mm, F.Cu at (210.8, 111.8)
- added D38: WS2812B, LED_SMD:LED_WS2812B_PLCC4_5.0x5.0mm_P3.2mm, F.Cu at (195.6, 111.8)
- added D39: WS2812B, LED_SMD:LED_WS2812B_PLCC4_5.0x5.0mm_P3.2mm, F.Cu at (210.8, 119.4)
- added D39: WS2812B, LED_SMD:LED_WS2812B_PLCC4_5.0x5.0mm_P3.2mm, F.Cu at (195.6, 119.4)
- added D4: WS2812B, LED_SMD:LED_WS2812B_PLCC4_5.0x5.0mm_P3.2mm, F.Cu at (134.6, 99.1)
- added D40: WS2812B, LED_SMD:LED_WS2812B_PLCC4_5.0x5.0mm_P3.2mm, F.Cu at (210.8, 127.0)
- added D40: WS2812B, LED_SMD:LED_WS2812B_PLCC4_5.0x5.0mm_P3.2mm, F.Cu at (195.6, 127.0)
- added D41: WS2812B, LED_SMD:LED_WS2812B_PLCC4_5.0x5.0mm_P3.2mm, F.Cu at (134.6, 132.1)
- added D42: WS2812B, LED_SMD:LED_WS2812B_PLCC4_5.0x5.0mm_P3.2mm, F.Cu at (134.6, 139.7)
- added D43: WS2812B, LED_SMD:LED_WS2812B_PLCC4_5.0x5.0mm_P3.2mm, F.Cu at (134.6, 147.3)
- added D44: WS2812B, LED_SMD:LED_WS2812B_PLCC4_5.0x5.0mm_P3.2mm, F.Cu at (134.6, 154.9)
- added D45: WS2812B, LED_SMD:LED_WS2812B_PLCC4_5.0x5.0mm_P3.2mm, F.Cu at (149.9, 132.1)
- added D46: WS2812B, LED_SMD:LED_WS2812B_PLCC4_5.0x5.0mm_P3.2mm, F.Cu at (149.9, 139.7)
- added D47: WS2812B, LED_SMD:LED_WS2812B_PLCC4_5.0x5.0mm_P3.2mm, F.Cu at (149.9, 147.3)
- added D48: WS2812B, LED_SMD:LED_WS2812B_PLCC4_5.0x5.0mm_P3.2mm, F.Cu at (149.9, 154.9)
- added D49: WS2812B, LED_SMD:LED_WS2812B_PLCC4_5.0x5.0mm_P3.2mm, F.Cu at (165.1, 132.1)
- added D5: WS2812B, LED_SMD:LED_WS2812B_PLCC4_5.0x5.0mm_P3.2mm, F.Cu at (149.9, 76.2)
- added D50: WS2812B, LED_SMD:LED_WS2812B_PLCC4_5.0x5.0mm_P3.2mm, F.Cu at (165.1, 139.7)
- added D51: WS2812B, LED_SMD:LED_WS2812B_PLCC4_5.0x5.0mm_P3.2mm, F.Cu at (165.1, 147.3)
- added D52: WS2812B, LED_SMD:LED_WS2812B_PLCC4_5.0x5.0mm_P3.2mm, F.Cu at (165.1, 154.9)
- added D53: WS2812B, LED_SMD:LED_WS2812B_PLCC4_5.0x5.0mm_P3.2mm, F.Cu at (180.3, 132.1)
- added D54: WS2812B, LED_SMD:LED_WS2812B_PLCC4_5.0x5.0mm_P3.2mm, F.Cu at (180.3, 139.7)
- added D55: WS2812B, LED_SMD:LED_WS2812B_PLCC4_5.0x5.0mm_P3.2mm, F.Cu at (180.3, 147.3)
- added D56: WS2812B, LED_SMD:LED_WS2812B_PLCC4_5.0x5.0mm_P3.2mm, F.Cu at (180.3, 154.9)
- added D57: WS2812B, LED_SMD:LED_WS2812B_PLCC4_5.0x5.0mm_P3.2mm, F.Cu at (210.8, 132.1)
- added D57: WS2812B, LED_SMD:LED_WS2812B_PLCC4_5.0x5.0mm_P3.2mm, F.Cu at (195.6, 132.1)
- added D58: WS2812B, LED_SMD:LED_WS2812B_PLCC4_5.0x5.0mm_P3.2mm, F.Cu at (210.8, 139.7)
- added D58: WS2812B, LED_SMD:LED_WS2812B_PLCC4_5.0x5.0mm_P3.2mm, F.Cu at (195.6, 139.7)
- added D59: WS2812B, LED_SMD:LED_WS2812B_PLCC4_5.0x5.0mm_P3.2mm, F.Cu at (210.8, 147.3)
- added D59: WS2812B, LED_SMD:LED_WS2812B_PLCC4_5.0x5.0mm_P3.2mm, F.Cu at (195.6, 147.3)
- added D6: WS2812B, LED_SMD:LED_WS2812B_PLCC4_5.0x5.0mm_P3.2mm, F.Cu at (149.9, 83.8)
- added D60: WS2812B, LED_SMD:LED_WS2812B_PLCC4_5.0x5.0mm_P3.2mm, F.Cu at (195.6, 154.9)
- added D60: WS2812B, LED_SMD:LED_WS2812B_PLCC4_5.0x5.0mm_P3.2mm, F.Cu at (210.8, 154.9)
- added D7: WS2812B, LED_SMD:LED_WS2812B_PLCC4_5.0x5.0mm_P3.2mm, F.Cu at (149.9, 91.4)
- added D8: WS2812B, LED_SMD:LED_WS2812B_PLCC4_5.0x5.0mm_P3.2mm, F.Cu at (149.9, 99.1)
- added D9: WS2812B, LED_SMD:LED_WS2812B_PLCC4_5.0x5.0mm_P3.2mm, F.Cu at (165.1, 76.2)
- added J1: Conn_01x02, Connector_PinHeader_2.54mm:PinHeader_1x02_P2.54mm_Vertical, B.Cu at (128.3, 74.9)
- added J10: Conn_01x02, Connector_PinHeader_2.54mm:PinHeader_1x02_P2.54mm_Vertical, B.Cu at (156.2, 74.9)
- added J100: Conn_01x02, Connector_PinHeader_2.54mm:PinHeader_1x02_P2.54mm_Vertical, B.Cu at (171.4, 138.4)
- added J101: Conn_01x02, Connector_PinHeader_2.54mm:PinHeader_1x02_P2.54mm_Vertical, B.Cu at (158.8, 146.1)
- added J102: Conn_01x02, Connector_PinHeader_2.54mm:PinHeader_1x02_P2.54mm_Vertical, B.Cu at (171.4, 146.1)
- added J103: Conn_01x02, Connector_PinHeader_2.54mm:PinHeader_1x02_P2.54mm_Vertical, B.Cu at (158.8, 153.7)
- added J104: Conn_01x02, Connector_PinHeader_2.54mm:PinHeader_1x02_P2.54mm_Vertical, B.Cu at (171.4, 153.7)
- added J105: Conn_01x02, Connector_PinHeader_2.54mm:PinHeader_1x02_P2.54mm_Vertical, B.Cu at (174.0, 130.8)
- added J106: Conn_01x02, Connector_PinHeader_2.54mm:PinHeader_1x02_P2.54mm_Vertical, B.Cu at (186.7, 130.8)
- added J107: Conn_01x02, Connector_PinHeader_2.54mm:PinHeader_1x02_P2.54mm_Vertical, B.Cu at (174.0, 138.4)
- added J108: Conn_01x02, Connector_PinHeader_2.54mm:PinHeader_1x02_P2.54mm_Vertical, B.Cu at (186.7, 138.4)
- added J109: Conn_01x02, Connector_PinHeader_2.54mm:PinHeader_1x02_P2.54mm_Vertical, B.Cu at (174.0, 146.1)
- added J11: Conn_01x02, Connector_PinHeader_2.54mm:PinHeader_1x02_P2.54mm_Vertical, B.Cu at (143.5, 82.5)
- added J110: Conn_01x02, Connector_PinHeader_2.54mm:PinHeader_1x02_P2.54mm_Vertical, B.Cu at (186.7, 146.1)
- added J111: Conn_01x02, Connector_PinHeader_2.54mm:PinHeader_1x02_P2.54mm_Vertical, B.Cu at (174.0, 153.7)
- added J112: Conn_01x02, Connector_PinHeader_2.54mm:PinHeader_1x02_P2.54mm_Vertical, B.Cu at (186.7, 153.7)
- added J113: Conn_01x02, Connector_PinHeader_2.54mm:PinHeader_1x02_P2.54mm_Vertical, B.Cu at (204.5, 130.8)
- added J113: Conn_01x02, Connector_PinHeader_2.54mm:PinHeader_1x02_P2.54mm_Vertical, B.Cu at (189.2, 130.8)
- added J114: Conn_01x02, Connector_PinHeader_2.54mm:PinHeader_1x02_P2.54mm_Vertical, B.Cu at (217.2, 130.8)
- added J114: Conn_01x02, Connector_PinHeader_2.54mm:PinHeader_1x02_P2.54mm_Vertical, B.Cu at (201.9, 130.8)
- added J115: Conn_01x02, Connector_PinHeader_2.54mm:PinHeader_1x02_P2.54mm_Vertical, B.Cu at (189.2, 138.4)
- added J115: Conn_01x02, Connector_PinHeader_2.54mm:PinHeader_1x02_P2.54mm_Vertical, B.Cu at (204.5, 138.4)
- added J116: Conn_01x02, Connector_PinHeader_2.54mm:PinHeader_1x02_P2.54mm_Vertical, B.Cu at (201.9, 138.4)
- added J116: Conn_01x02, Connector_PinHeader_2.54mm:PinHeader_1x02_P2.54mm_Vertical, B.Cu at (217.2, 138.4)
- added J117: Conn_01x02, Connector_PinHeader_2.54mm:PinHeader_1x02_P2.54mm_Vertical, B.Cu at (204.5, 146.1)
- added J117: Conn_01x02, Connector_PinHeader_2.54mm:PinHeader_1x02_P2.54mm_Vertical, B.Cu at (189.2, 146.1)
- added J118: Conn_01x02, Connector_PinHeader_2.54mm:PinHeader_1x02_P2.54mm_Vertical, B.Cu at (201.9, 146.1)
- added J118: Conn_01x02, Connector_PinHeader_2.54mm:PinHeader_1x02_P2.54mm_Vertical, B.Cu at (217.2, 146.1)
- added J119: Conn_01x02, Connector_PinHeader_2.54mm:PinHeader_1x02_P2.54mm_Vertical, B.Cu at (189.2, 153.7)
- added J119: Conn_01x02, Connector_PinHeader_2.54mm:PinHeader_1x02_P2.54mm_Vertical, B.Cu at (204.5, 153.7)
- added J12: Conn_01x02, Connector_PinHeader_2.54mm:PinHeader_1x02_P2.54mm_Vertical, B.Cu at (156.2, 82.5)
- added J120: Conn_01x02, Connector_PinHeader_2.54mm:PinHeader_1x02_P2.54mm_Vertical, B.Cu at (201.9, 153.7)
- added J120: Conn_01x02, Connector_PinHeader_2.54mm:PinHeader_1x02_P2.54mm_Vertical, B.Cu at (217.2, 153.7)
- added J13: Conn_01x02, Connector_PinHeader_2.54mm:PinHeader_1x02_P2.54mm_Vertical, B.Cu at (143.5, 90.2)
- added J14: Conn_01x02, Connector_PinHeader_2.54mm:PinHeader_1x02_P2.54mm_Vertical, B.Cu at (156.2, 90.2)
- added J15: Conn_01x02, Connector_PinHeader_2.54mm:PinHeader_1x02_P2.54mm_Vertical, B.Cu at (143.5, 97.8)
- added J16: Conn_01x02, Connector_PinHeader_2.54mm:PinHeader_1x02_P2.54mm_Vertical, B.Cu at (156.2, 97.8)
- added J17: Conn_01x02, Connector_PinHeader_2.54mm:PinHeader_1x02_P2.54mm_Vertical, B.Cu at (158.8, 74.9)
- added J18: Conn_01x02, Connector_PinHeader_2.54mm:PinHeader_1x02_P2.54mm_Vertical, B.Cu at (171.4, 74.9)
- added J19: Conn_01x02, Connector_PinHeader_2.54mm:PinHeader_1x02_P2.54mm_Vertical, B.Cu at (158.8, 82.5)
- added J2: Conn_01x02, Connector_PinHeader_2.54mm:PinHeader_1x02_P2.54mm_Vertical, B.Cu at (141.0, 74.9)
- added J20: Conn_01x02, Connector_PinHeader_2.54mm:PinHeader_1x02_P2.54mm_Vertical, B.Cu at (171.4, 82.5)
- added J21: Conn_01x02, Connector_PinHeader_2.54mm:PinHeader_1x02_P2.54mm_Vertical, B.Cu at (158.8, 90.2)
- added J22: Conn_01x02, Connector_PinHeader_2.54mm:PinHeader_1x02_P2.54mm_Vertical, B.Cu at (171.4, 90.2)
- added J23: Conn_01x02, Connector_PinHeader_2.54mm:PinHeader_1x02_P2.54mm_Vertical, B.Cu at (158.8, 97.8)
- added J24: Conn_01x02, Connector_PinHeader_2.54mm:PinHeader_1x02_P2.54mm_Vertical, B.Cu at (171.4, 97.8)
- added J25: Conn_01x02, Connector_PinHeader_2.54mm:PinHeader_1x02_P2.54mm_Vertical, B.Cu at (174.0, 74.9)
- added J26: Conn_01x02, Connector_PinHeader_2.54mm:PinHeader_1x02_P2.54mm_Vertical, B.Cu at (186.7, 74.9)
- added J27: Conn_01x02, Connector_PinHeader_2.54mm:PinHeader_1x02_P2.54mm_Vertical, B.Cu at (174.0, 82.5)
- added J28: Conn_01x02, Connector_PinHeader_2.54mm:PinHeader_1x02_P2.54mm_Vertical, B.Cu at (186.7, 82.5)
- added J29: Conn_01x02, Connector_PinHeader_2.54mm:PinHeader_1x02_P2.54mm_Vertical, B.Cu at (174.0, 90.2)
- added J3: Conn_01x02, Connector_PinHeader_2.54mm:PinHeader_1x02_P2.54mm_Vertical, B.Cu at (128.3, 82.5)
- added J30: Conn_01x02, Connector_PinHeader_2.54mm:PinHeader_1x02_P2.54mm_Vertical, B.Cu at (186.7, 90.2)
- added J31: Conn_01x02, Connector_PinHeader_2.54mm:PinHeader_1x02_P2.54mm_Vertical, B.Cu at (174.0, 97.8)
- added J32: Conn_01x02, Connector_PinHeader_2.54mm:PinHeader_1x02_P2.54mm_Vertical, B.Cu at (186.7, 97.8)
- added J33: Conn_01x02, Connector_PinHeader_2.54mm:PinHeader_1x02_P2.54mm_Vertical, B.Cu at (204.5, 74.9)
- added J33: Conn_01x02, Connector_PinHeader_2.54mm:PinHeader_1x02_P2.54mm_Vertical, B.Cu at (189.2, 74.9)
- added J34: Conn_01x02, Connector_PinHeader_2.54mm:PinHeader_1x02_P2.54mm_Vertical, B.Cu at (217.2, 74.9)
- added J34: Conn_01x02, Connector_PinHeader_2.54mm:PinHeader_1x02_P2.54mm_Vertical, B.Cu at (201.9, 74.9)
- added J35: Conn_01x02, Connector_PinHeader_2.54mm:PinHeader_1x02_P2.54mm_Vertical, B.Cu at (204.5, 82.5)
- added J35: Conn_01x02, Connector_PinHeader_2.54mm:PinHeader_1x02_P2.54mm_Vertical, B.Cu at (189.2, 82.5)
- added J36: Conn_01x02, Connector_PinHeader_2.54mm:PinHeader_1x02_P2.54mm_Vertical, B.Cu at (201.9, 82.5)
- added J36: Conn_01x02, Connector_PinHeader_2.54mm:PinHeader_1x02_P2.54mm_Vertical, B.Cu at (217.2, 82.5)
- added J37: Conn_01x02, Connector_PinHeader_2.54mm:PinHeader_1x02_P2.54mm_Vertical, B.Cu at (204.5, 90.2)
- added J37: Conn_01x02, Connector_PinHeader_2.54mm:PinHeader_1x02_P2.54mm_Vertical, B.Cu at (189.2, 90.2)
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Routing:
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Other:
- board size 91.4 x 81.3 mm -> 91.4 x 83.8 mm
